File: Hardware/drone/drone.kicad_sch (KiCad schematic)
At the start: 9 parts, among them M1 Motor_DC, M2 Motor_DC, M3 Motor_DC, M4 Motor_DC, U1 ESP32-DEVKITC, U2 MPU6050 DevKit, U3 HW_611, U4 DRV8833, U5 DRV8833

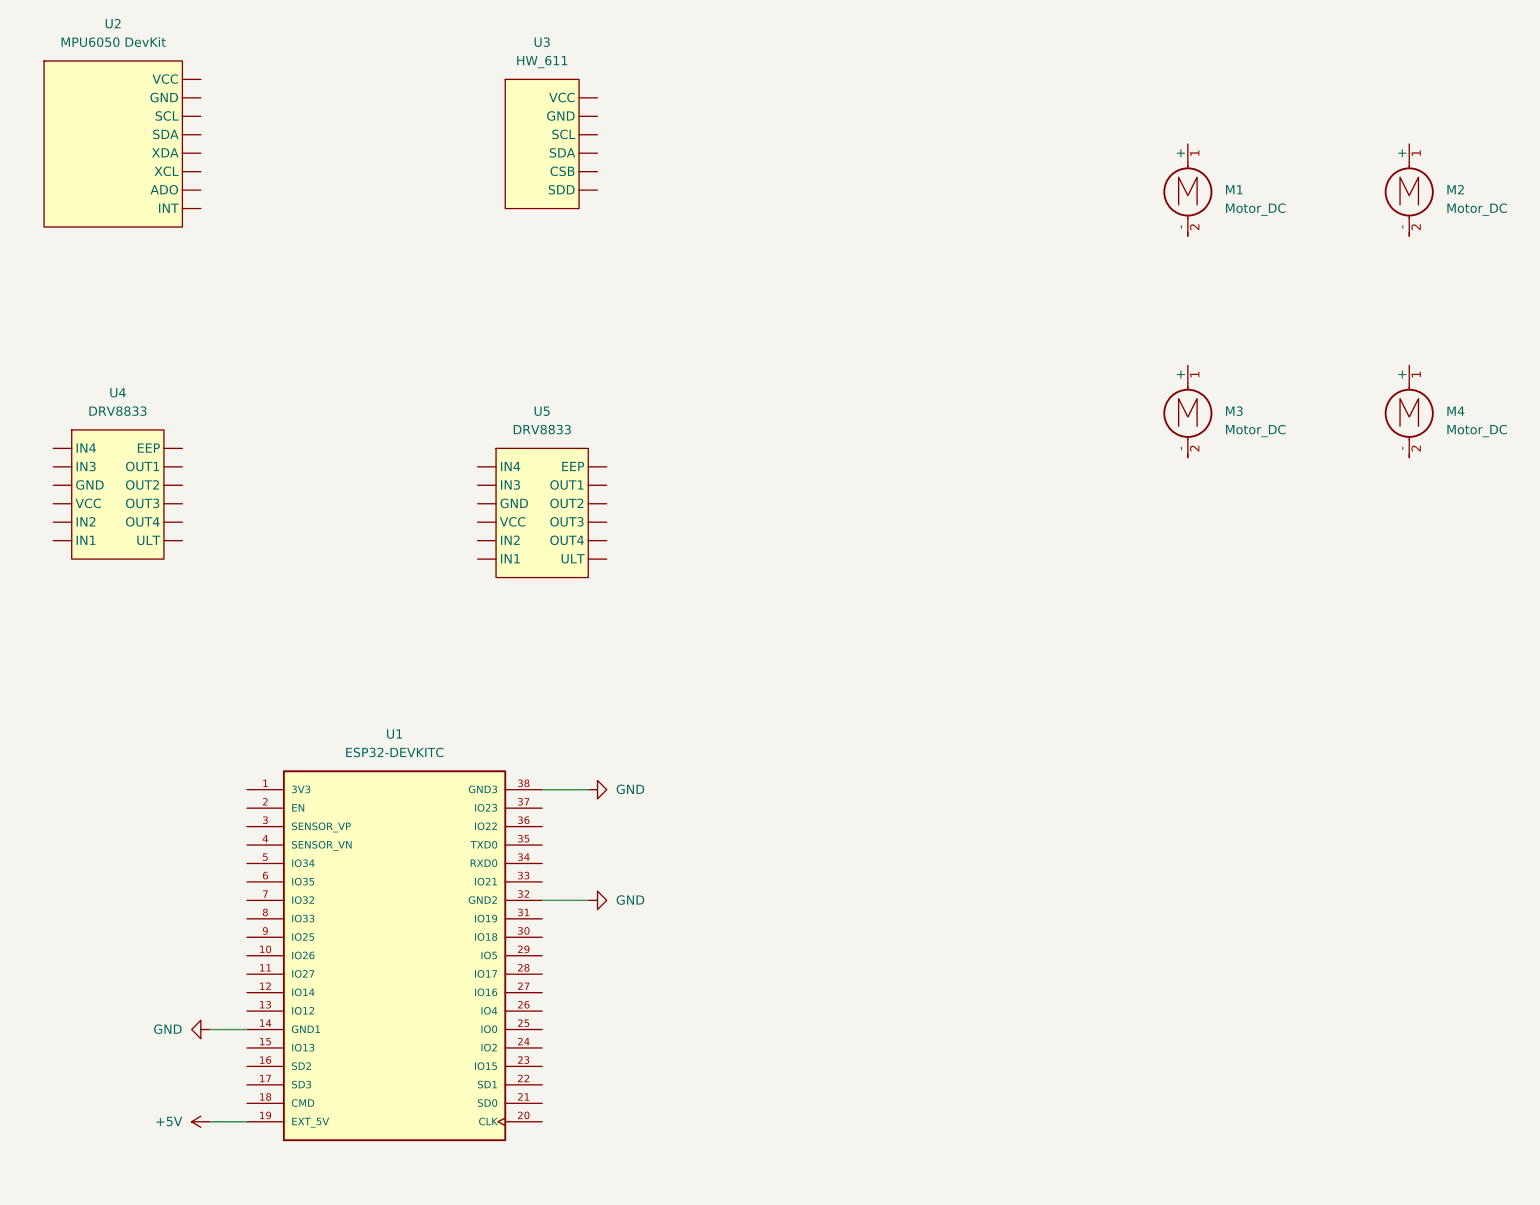
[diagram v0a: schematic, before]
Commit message: Hardware schematic update.
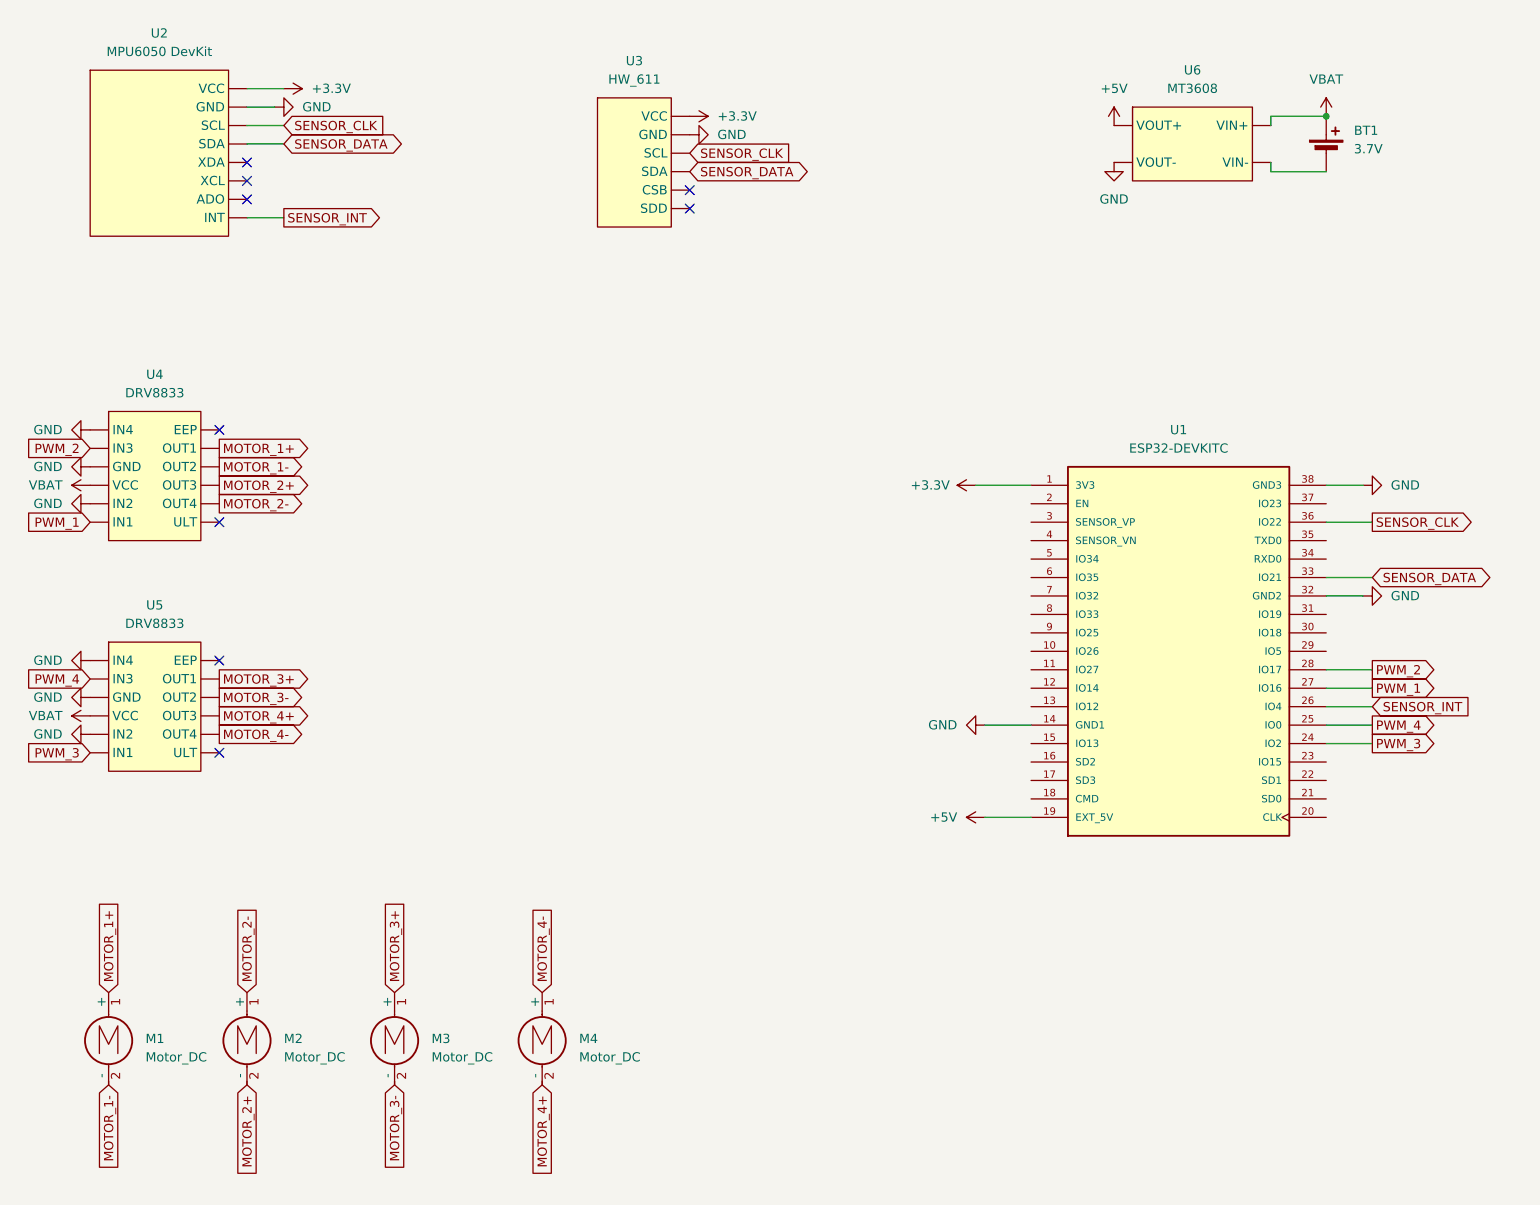
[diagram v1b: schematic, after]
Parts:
- added BT1: 3.7V, symbol Device:Battery_Cell
- added U6: MT3608, symbol Custom_drone:MT3608
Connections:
- net +5V: now also U6. (VIN-)
- net GND: now also U2. (INT), U3. (SDD), U4. (ULT), U5. (ULT), U6. (VIN-)
- net MOTOR_3+: now reaches M3.1 (+)
- net MOTOR_3+: now also U5. (ULT)
- net MOTOR_3-: now reaches M3.2 (-)
- net MOTOR_3-: now also U5. (ULT)
- net SENSOR_DATA: now reaches U3. (SDD)
- net SENSOR_DATA: now also U1.33 (IO21), U2. (INT)
- net MOTOR_4-: now reaches M4.1 (+)
- net MOTOR_4-: now also U5. (ULT)
- net MOTOR_4+: now reaches M4.2 (-)
- net MOTOR_4+: now also U5. (ULT)
- net MOTOR_1+: now reaches M1.1 (+)
- net MOTOR_1+: now also U4. (ULT)
- net MOTOR_1-: now reaches M1.2 (-)
- net MOTOR_1-: now also U4. (ULT)
- net VBAT: now reaches U4. (ULT)
- net VBAT: now also U5. (ULT), BT1.1 (+), U6. (VIN-)
- net SENSOR_INT: now reaches U2. (INT)
- net SENSOR_INT: now also U1.26 (IO4)
- net MOTOR_2-: now reaches M2.1 (+)
- net MOTOR_2-: now also U4. (ULT)
- net MOTOR_2+: now reaches M2.2 (-)
- net MOTOR_2+: now also U4. (ULT)
- net +3.3V: now reaches U1.1 (3V3)
- net +3.3V: now also U2. (INT), U3. (SDD)
- net PWM_3: now reaches U1.24 (IO2)
- net PWM_3: now also U5. (ULT)
- net PWM_4: now reaches U1.25 (IO0)
- net PWM_4: now also U5. (ULT)
- net PWM_1: now reaches U1.27 (IO16)
- net PWM_1: now also U4. (ULT)
- net PWM_2: now reaches U1.28 (IO17)
- net PWM_2: now also U4. (ULT)
- net SENSOR_CLK: now reaches U1.36 (IO22)
- net SENSOR_CLK: now also U2. (INT), U3. (SDD)
- new net: BT1.2 (-), U6. (VIN-)
- no-connect marks 0 -> 9
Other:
- moved on the sheet: M1, M2, M3, M4, U1, U2, U3, U4, U5
